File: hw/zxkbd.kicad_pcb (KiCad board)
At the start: 2 copper layers, 148 x 48 mm, 55 parts, among them J1 TAPE, J3 AY_IN, J4 SCART, J5 SERIAL, J6 ISP, Q1 BC846, SW1 RESET, SW2 MAGIC, SW3 AVR_RST, U1 74HC373, U10 74HC373, U11 PS2CONN, U12 ATmega328P-AU, U13 74HC373, U14 74HC373, U15 74HC373, U16 74HC373, U2 74HC30, U3 74HC30, U4 74HC30, U5 74HC30, U6 74HC30, U7 74HC373, U8 pentagon_conn, U9 74HC373, Y1 14.7456

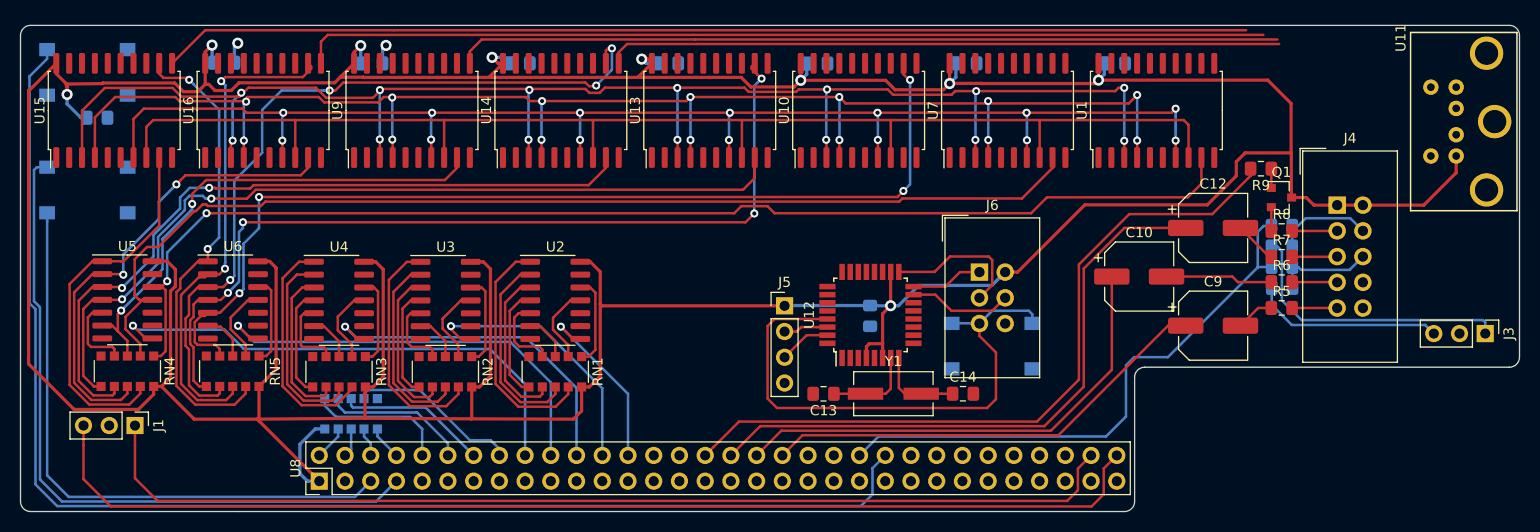
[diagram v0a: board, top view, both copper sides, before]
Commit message: PCB first pass
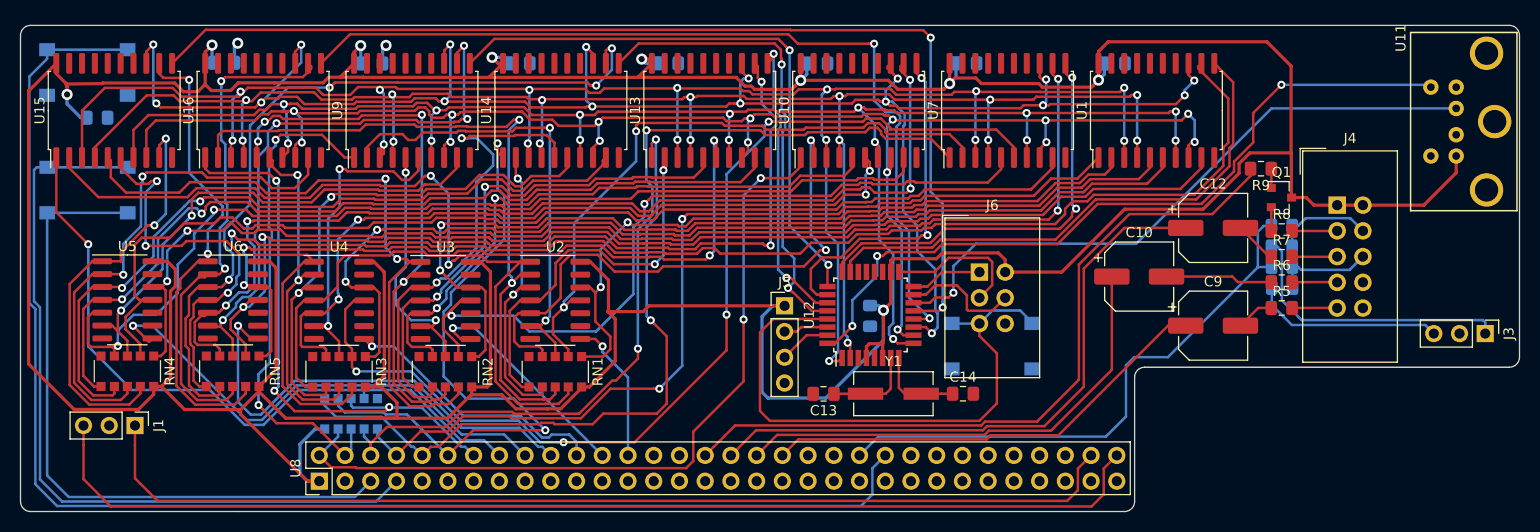
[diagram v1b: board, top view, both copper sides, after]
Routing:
- net /D4: track 0.00 -> 183.7 mm, vias 0 -> 17
- net /KDA4: track 8.83 -> 128.7 mm, vias 0 -> 2
- net /KDB4: track 7.84 -> 112.5 mm, vias 0 -> 4
- net /KDB2: track 7.78 -> 103.0 mm, vias 0 -> 4
- net /KDA2: track 8.89 -> 100.4 mm, vias 0 -> 2
- net /KDD3: track 7.77 -> 99.1 mm, vias 0 -> 2
- net /KA0: track 3.39 -> 93.5 mm, vias 0 -> 2
- net /KA1: track 2.88 -> 89.2 mm, vias 0 -> 2
- net /KDA1: track 9.02 -> 92.0 mm, vias 0 -> 2
- net /PCLK: track 0.00 -> 75.1 mm, vias 0 -> 3
- net /KA3: track 3.38 -> 77.1 mm, vias 0 -> 2
- net /KDB1: track 7.90 -> 77.3 mm, vias 0 -> 2
- net /KDD2: track 7.64 -> 75.6 mm, vias 0 -> 4
- net /PDATA: track 0.00 -> 63.1 mm, vias 0 -> 1
- net /KDA0: track 8.98 -> 70.6 mm, vias 0 -> 2
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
